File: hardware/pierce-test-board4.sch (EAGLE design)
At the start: 8 parts

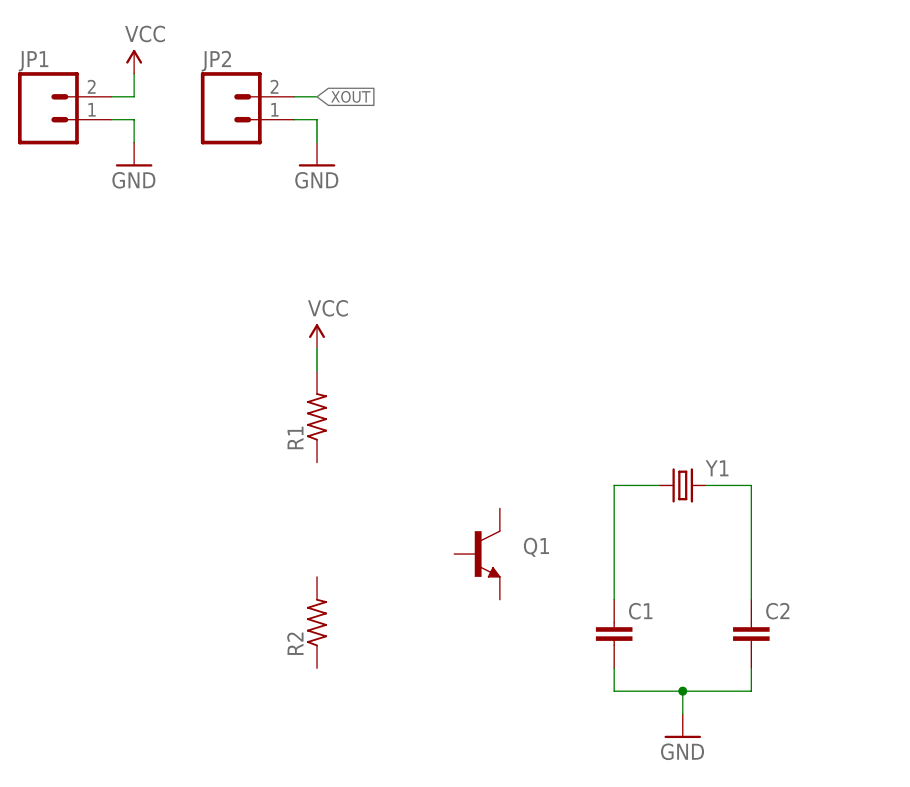
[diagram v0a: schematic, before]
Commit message: yet another test pcb
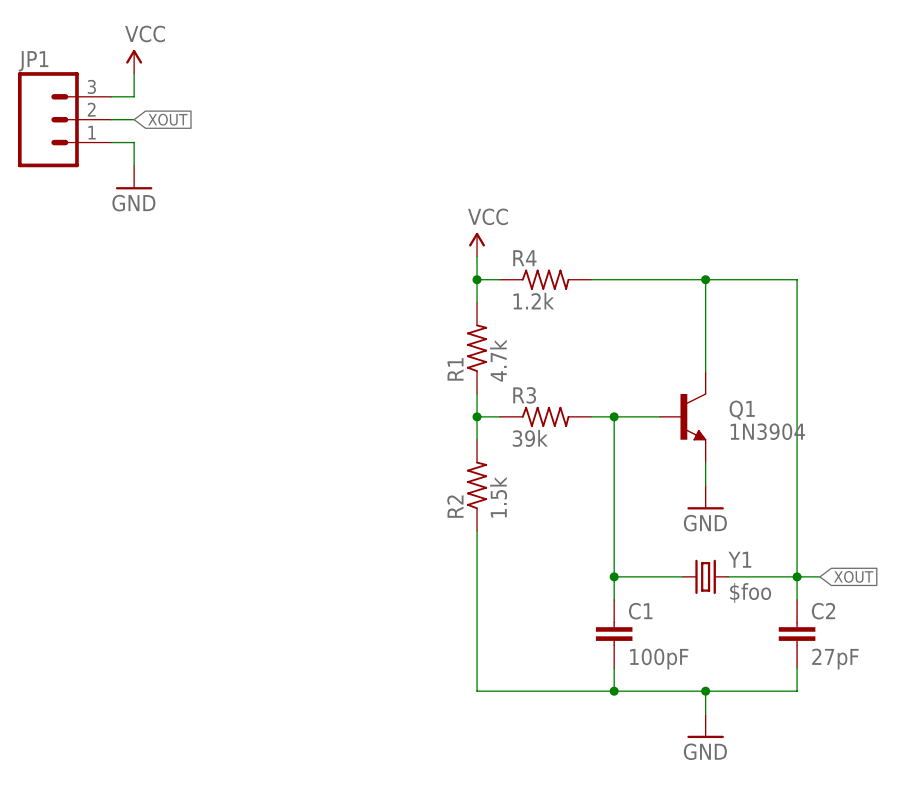
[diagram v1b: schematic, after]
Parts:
- removed JP2: M02PTH, A_butts:M02PTH
- added R3: 39k, A_butts:RESISTORPTH-AXIAL-5.08MM
- added R4: 1.2k, A_butts:RESISTORPTH-AXIAL-5.08MM
- C1: value (none) -> 100pF
- C2: value (none) -> 27pF
- JP1: value M02PTH -> (none); device A_butts:M02PTH -> A_butts:M03PTH
- Q1: value (none) -> 1N3904
- R1: value (none) -> 4.7k
- R2: value (none) -> 1.5k
- Y1: value (none) -> $foo
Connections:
- removed net N$1: C2.1, Y1.2
- new net N$2: R1.1, R2.2, R3.1
- net GND: now also Q1.E, R2.1; no longer JP2.1
- net N$4: now also Q1.B, R3.2
- net VCC: now also JP1.3, R4.1; no longer JP1.2
- net XOUT: now also C2.1, JP1.2, Q1.C, R4.2, Y1.2; no longer JP2.2
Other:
- moved on the sheet: C2, Q1, R1, R2, Y1
